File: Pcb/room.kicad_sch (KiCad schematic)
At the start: 38 parts, among them J1 USB_C_Receptacle_USB2.0_14P, J2 Screw_Terminal_01x10, J3 BOOT, J4 Screw_Terminal_01x03, K1 D1, K2 D2, K3 D3, K4 D4, Q1 BC547, Q2 BC547, Q3 BC547, Q4 BC547, SW1 SW_Push, U1 ESP32-C3-WROOM-02, U2 AMS1117-3.3

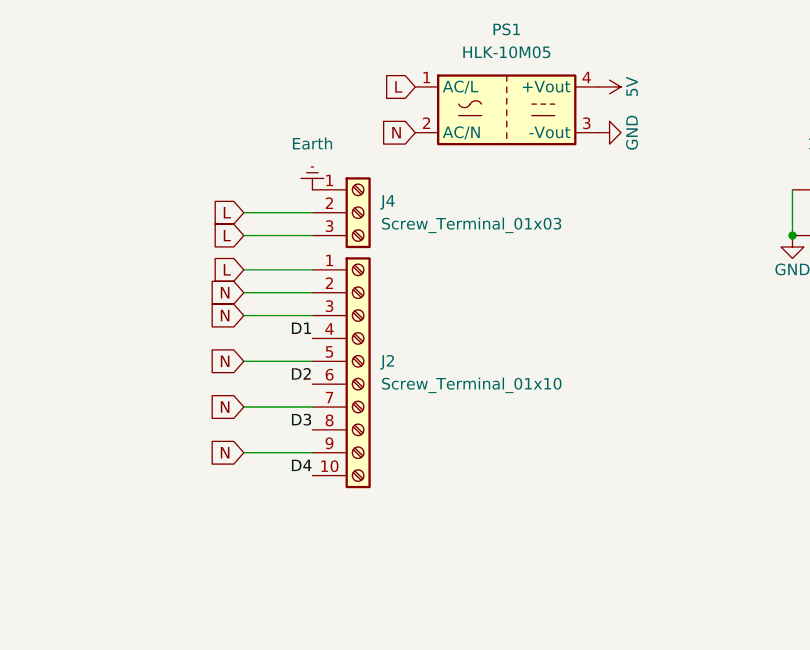
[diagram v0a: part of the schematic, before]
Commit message: Mostly done
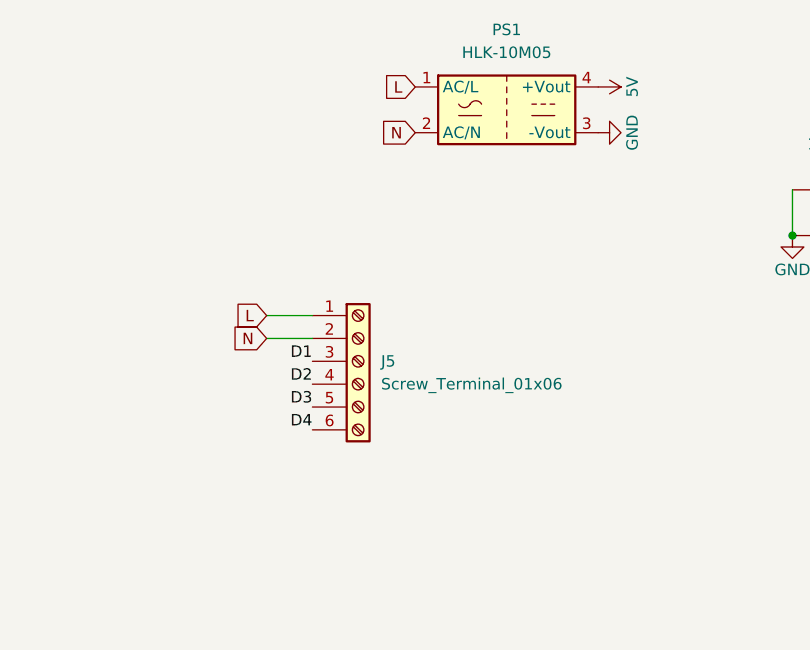
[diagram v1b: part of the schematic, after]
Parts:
- removed J2: Screw_Terminal_01x10, TerminalBlock:TerminalBlock_Xinya_XY308-2.54-10P_1x10_P2.54mm_Horizontal, symbol Connector:Screw_Terminal_01x10
- removed J4: Screw_Terminal_01x03, TerminalBlock:TerminalBlock_Xinya_XY308-2.54-3P_1x03_P2.54mm_Horizontal, symbol Connector:Screw_Terminal_01x03
- added J5: Screw_Terminal_01x06, TerminalBlock:TerminalBlock_bornier-6_P5.08mm, symbol Connector:Screw_Terminal_01x06
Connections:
- net D1: now also J5.3 (Pin_3)
- net D2: now also J5.4 (Pin_4)
- net D3: now also J5.5 (Pin_5)
- net D4: now also J5.6 (Pin_6)
- net L: now also J5.1 (Pin_1)
- net N: now also J5.2 (Pin_2)
